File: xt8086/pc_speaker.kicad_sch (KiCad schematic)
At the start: 7 parts, among them J5 SJ1-3525N, Q1 2N7000, U3 CMT-7525-80-SMT-TR

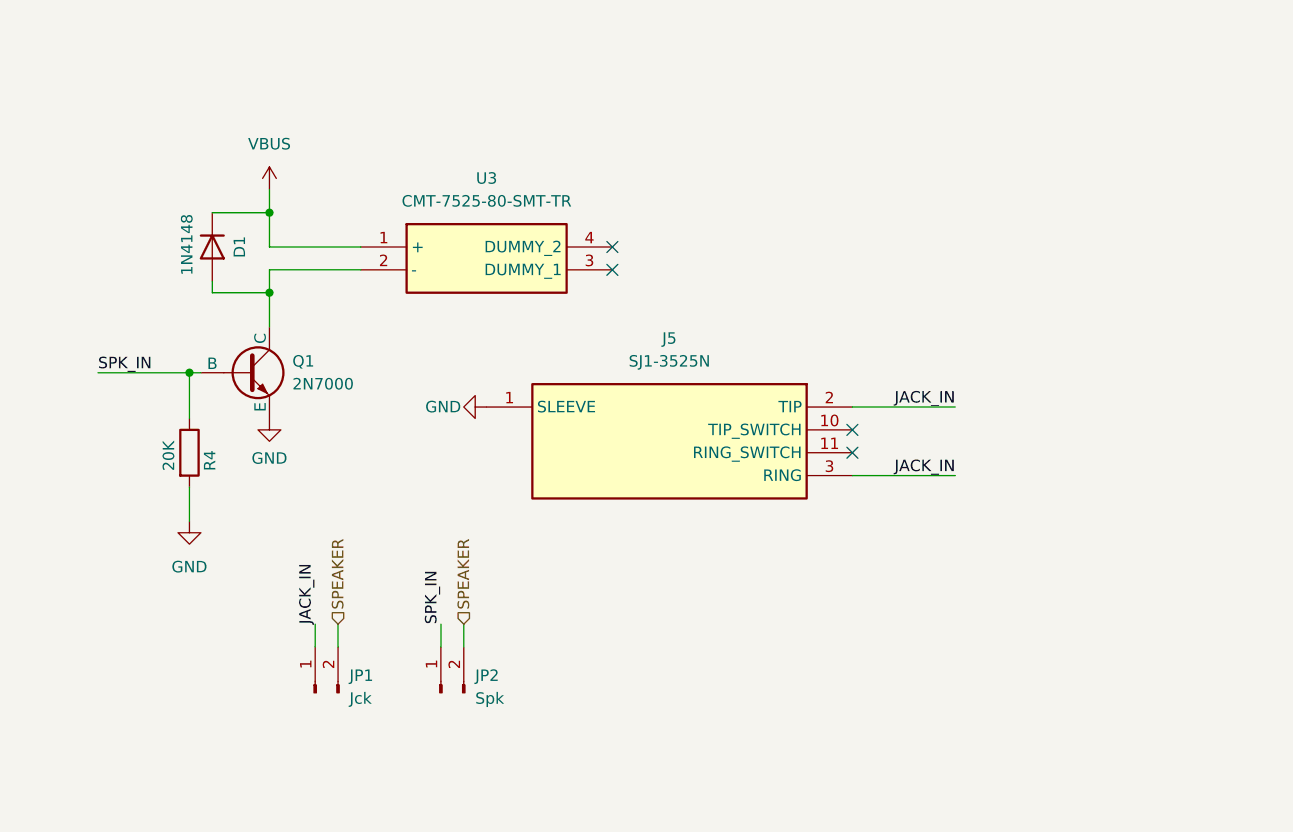
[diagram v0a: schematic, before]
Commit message: Board updates
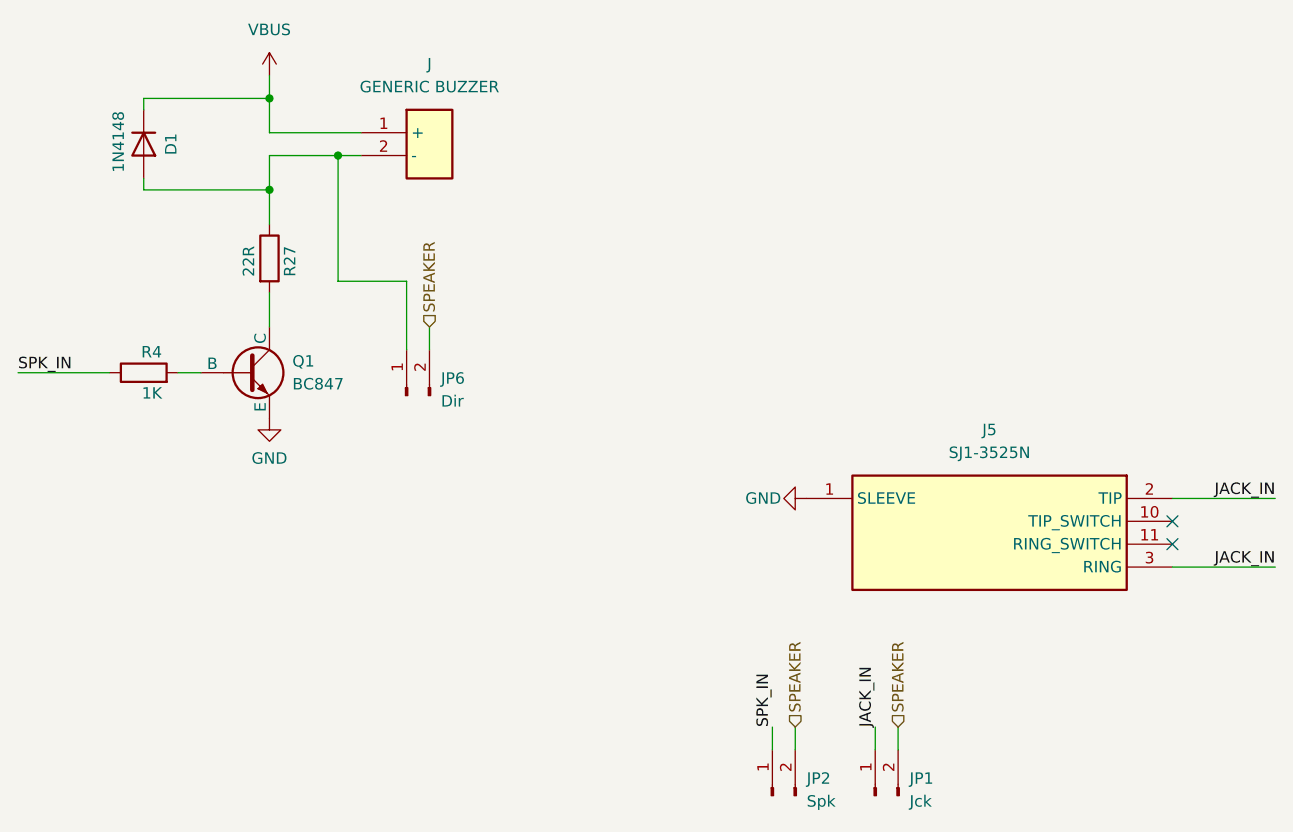
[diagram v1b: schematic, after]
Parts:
- added JP6: Dir, Jumper:SolderJumper-2_P1.3mm_Open_Pad1.0x1.5mm, symbol xt8086:Conn_01x02_Pin
- added R27: 22R, xt8086:R_0805_2012Metric, symbol xt8086:R
- J: renamed from U3; value CMT-7525-80-SMT-TR -> GENERIC BUZZER
- Q1: value 2N7000 -> BC847
- R4: value 20K -> 1K
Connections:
- net GND: no longer R4.2
- net SPEAKER: now also JP6.2 (Pin_2)
- net SPK_IN: no longer Q1.2 (B)
- net at D1.2 (A), J.2 (-): now also JP6.1 (Pin_1), R27.1; no longer Q1.1 (C)
- new net: Q1.1 (C), R27.2
- new net: Q1.2 (B), R4.2
- no-connect marks 4 -> 2
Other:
- moved on the sheet: D1, J5, JP1, JP2
